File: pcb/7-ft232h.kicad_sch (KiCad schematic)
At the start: 29 parts, among them U701 FT232HL, U702 93LC56BT-I/OT, Y701 12MHz ABM8-272-T3

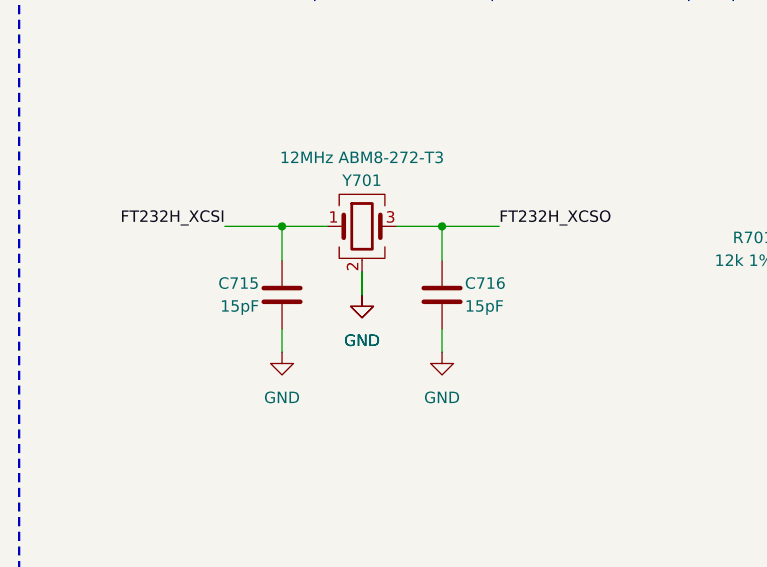
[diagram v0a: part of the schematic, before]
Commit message: route more scsi traces
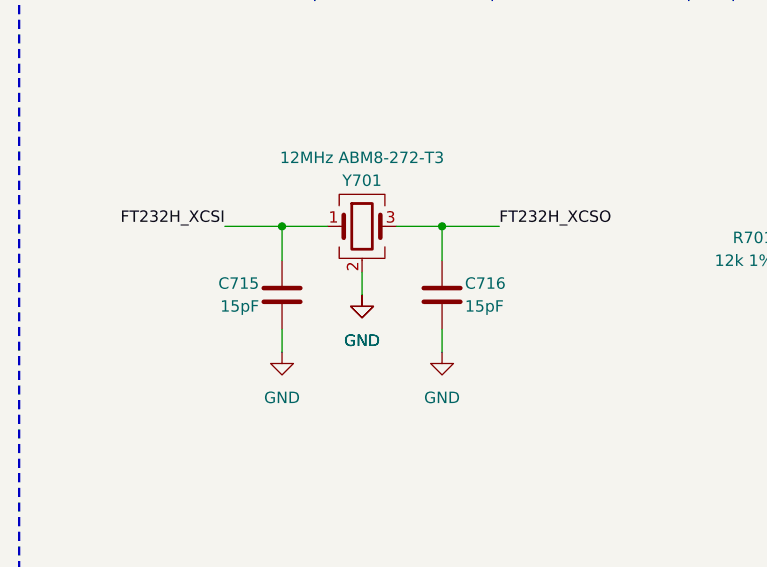
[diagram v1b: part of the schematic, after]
